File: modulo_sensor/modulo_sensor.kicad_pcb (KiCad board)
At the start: 2 copper layers, 112.4 x 36.6 mm, 33 parts, among them J1 Conn_01x08_Pin, U1 74HC14DR2G

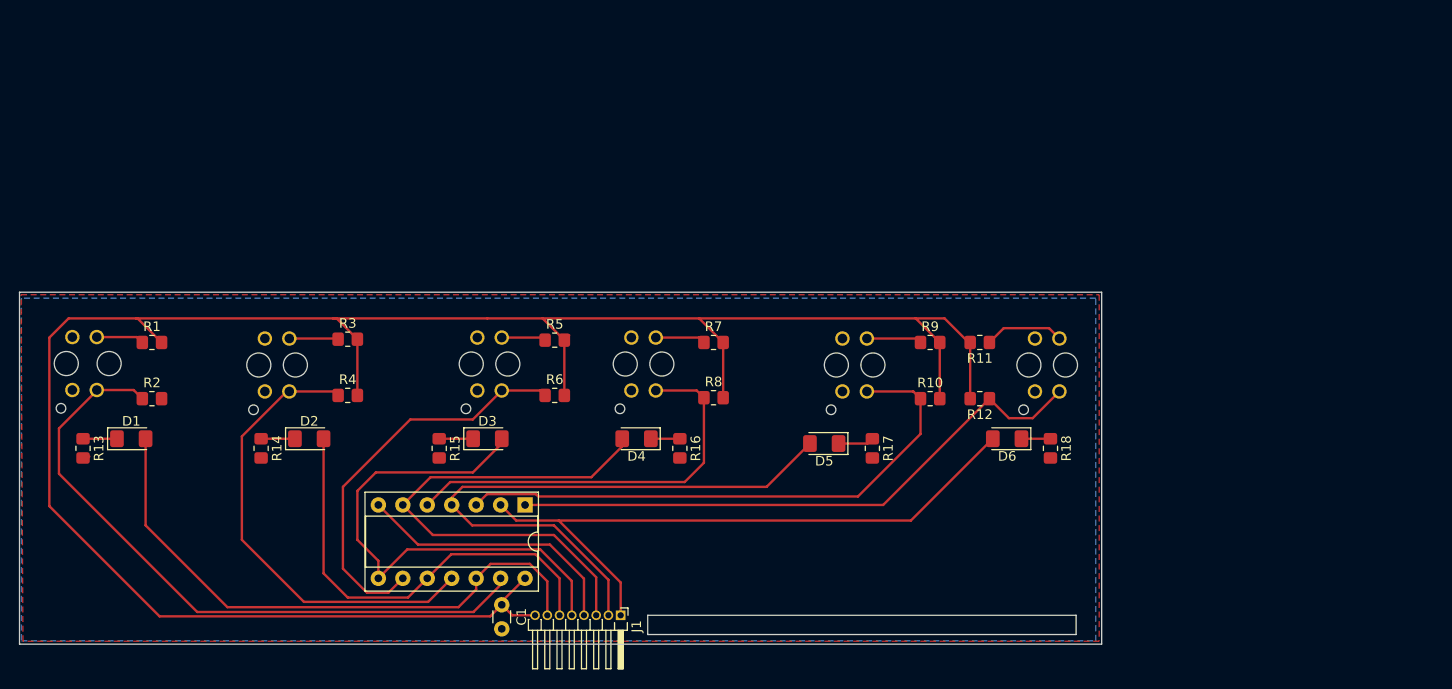
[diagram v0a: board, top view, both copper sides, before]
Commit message: feat: Placa doble faz
Placa 120x30mm doble faz
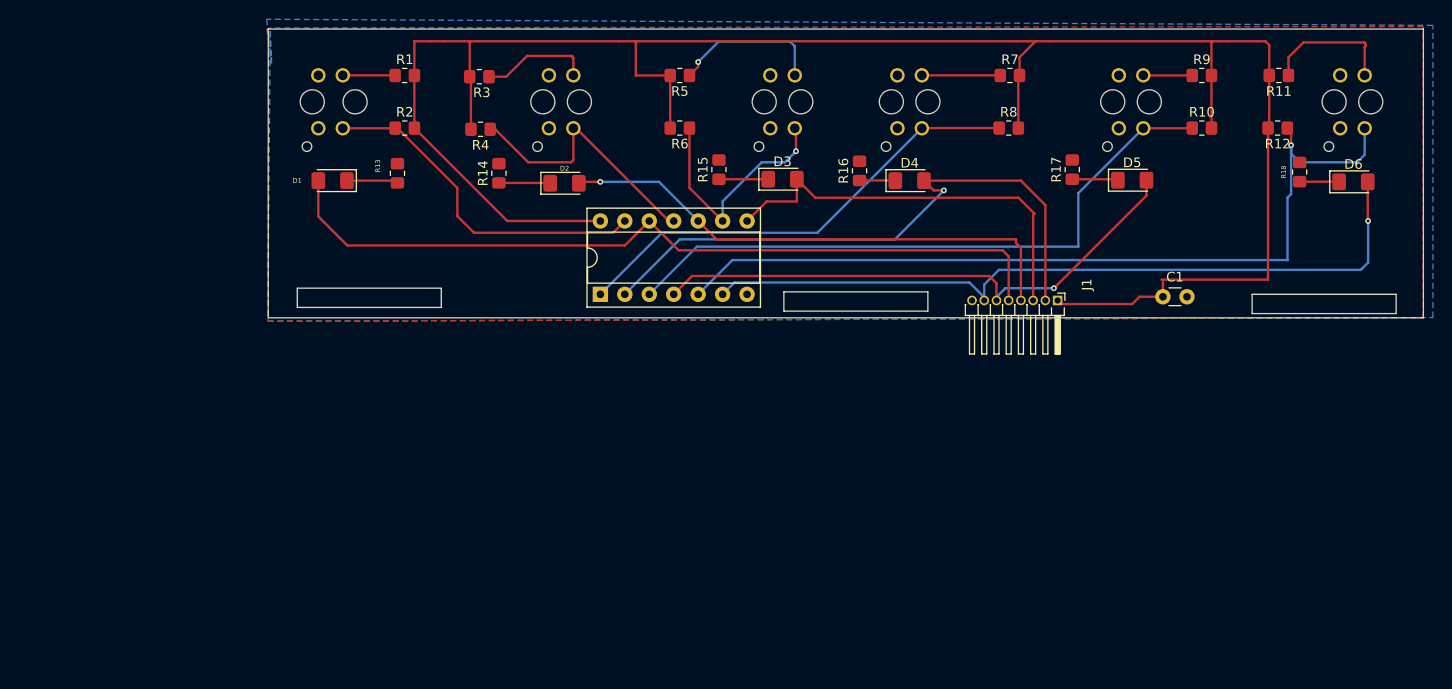
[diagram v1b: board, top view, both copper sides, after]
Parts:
- moved C1 75.8 mm to (161.2, 55.8), turned to 0 degrees
- moved J1 55.9 mm to (150.2, 56.1)
- moved D6 44.8 mm to (181.0, 43.8), turned to 0 degrees
- moved R13 43.4 mm to (81.7, 42.9), turned to 90 degrees
- moved D5 42.1 mm to (158.0, 43.6), turned to 0 degrees
- moved Sensor6 41.9 mm to (180.9, 35.5)
- moved R12 41.8 mm to (173.1, 38.2)
- moved R11 41.6 mm to (173.2, 32.8)
- moved R8 41.5 mm to (145.2, 38.2)
- moved R7 41.4 mm to (145.3, 32.8)
- moved R15 41.0 mm to (115.1, 42.5), turned to 90 degrees
- moved Sensor3 40.8 mm to (121.7, 35.5)
- moved D3 40.8 mm to (121.7, 43.5)
- moved Sensor2 40.2 mm to (98.7, 35.5)
- moved R10 39.8 mm to (165.2, 38.2)
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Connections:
- J1 pad 1: /Led_Sensor6 -> vcc
- J1 pad 2: /Led_Sensor5 -> /Led_Sensor4
- J1 pad 3: /Led_Sensor4 -> /Led_Sensor3
- J1 pad 4: GND -> /Led_Sensor2
- J1 pad 5: /Led_Sensor3 -> /Led_Sensor1
- J1 pad 6: /Led_Sensor2 -> /Led_Sensor5
- J1 pad 7: /Led_Sensor1 -> /Led_Sensor6
- J1 pad 8: vcc -> GND
- U1 pad 1: /Sensor6 -> /Sensor4
- U1 pad 2: /Led_Sensor6 -> /Led_Sensor4
- U1 pad 5: /Sensor4 -> /Sensor6
- U1 pad 6: /Led_Sensor4 -> /Led_Sensor6
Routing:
- net /Sensor1: track 69.6 -> 36.7 mm
- net GND: track 30.2 -> 0.18 mm
- net /Sensor6: track 62.1 -> 88.7 mm, vias 0 -> 1
- net /Led_Sensor1: track 61.1 -> 84.2 mm
- net /Sensor2: track 48.3 -> 27.9 mm
- net /Sensor3: track 41.7 -> 25.3 mm, vias 0 -> 1
- net /Led_Sensor6: track 67.7 -> 81.0 mm, vias 0 -> 1
- net vcc: track 222.6 -> 210.5 mm
- net Net-(R5-Pad1): track 4.61 -> 15.9 mm, vias 0 -> 1
- net /Led_Sensor4: track 53.3 -> 64.1 mm, vias 0 -> 1
- net /Led_Sensor3: track 53.2 -> 43.9 mm
- net /Led_Sensor2: track 46.3 -> 54.9 mm, vias 0 -> 1
- net /Sensor5: track 59.0 -> 66.8 mm
- net Net-(R3-Pad1): track 5.10 -> 11.6 mm
- net /Sensor4: track 42.6 -> 48.6 mm
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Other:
- board size 112.4 x 36.6 mm -> 120 x 30 mm
